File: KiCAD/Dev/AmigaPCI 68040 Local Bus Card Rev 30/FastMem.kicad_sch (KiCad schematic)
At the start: 29 parts, among them CN400 SPI, U400 ICE40HX1K-VQ100, U400F1 W25X20CLSN, U401 SDRAM(16Mx32), U402 SDRAM(16Mx32)

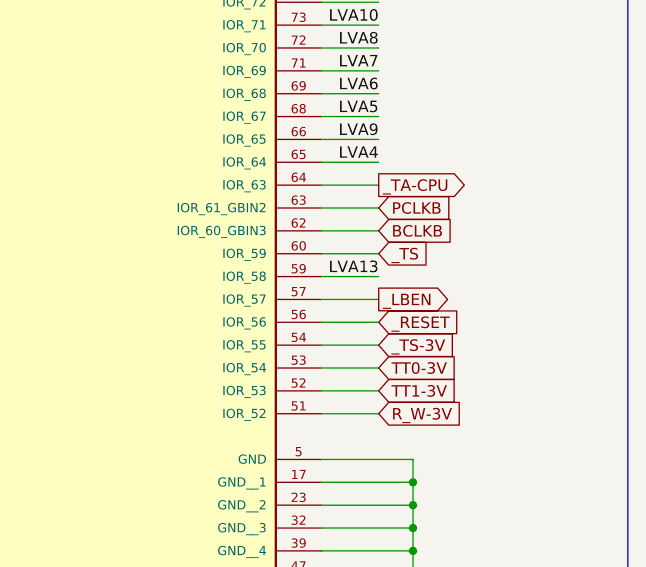
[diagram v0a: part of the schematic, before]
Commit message: CPU Local Bus Card Rev 3.0 Routing 18-JUL-2024
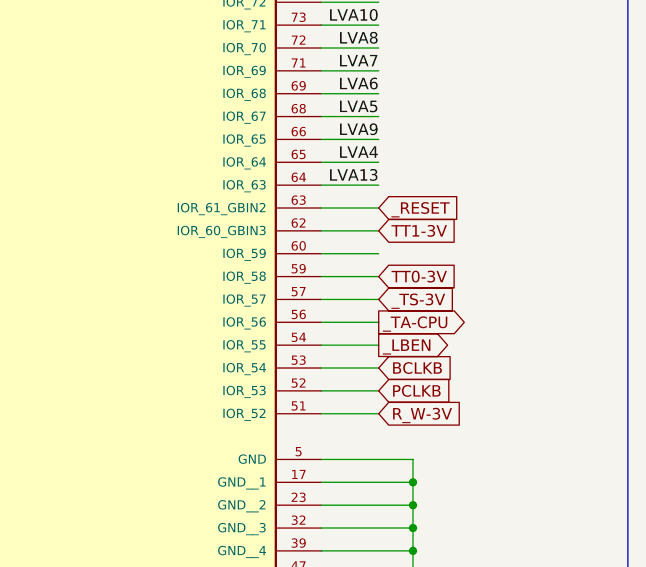
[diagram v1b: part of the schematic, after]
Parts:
- CN400: footprint Connector_PinHeader_2.54mm:PinHeader_2x03_P2.54mm_Vertical -> Connector_PinHeader_2.54mm:PinHeader_1x06_P2.54mm_Vertical
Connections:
- net BCLKB: now also U400.53 (IOR_54); no longer U400.62 (IOR_60_GBIN3)
- net LVA13: now also U400.64 (IOR_63); no longer U400.59 (IOR_58)
- net PCLKB: now also U400.52 (IOR_53); no longer U400.63 (IOR_61_GBIN2)
- net TT0-3V: now also U400.59 (IOR_58); no longer U400.53 (IOR_54)
- net TT1-3V: now also U400.62 (IOR_60_GBIN3); no longer U400.52 (IOR_53)
- net _LBEN: now also U400.54 (IOR_55); no longer U400.57 (IOR_57)
- net _RESET: now also U400.63 (IOR_61_GBIN2); no longer U400.56 (IOR_56)
- net _TA-CPU: now also U400.56 (IOR_56); no longer U400.64 (IOR_63)
- net _TS-3V: now also U400.57 (IOR_57); no longer U400.54 (IOR_55)
- net _TS: no longer names the net of U400.60 (IOR_59)
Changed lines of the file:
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@@
 	)
 	(label "LVA13"
-		(at 383.54 179.07 180)
+		(at 383.54 168.91 180)
 		(fields_autoplaced yes)
 		(effects
@@
 	(global_label "PCLKB"
 		(shape input)
-		(at 383.54 171.45 0)
+		(at 383.54 191.77 0)
 		(fields_autoplaced yes)
 		(effects
@@
 		)
 		(property "Intersheetrefs" "${INTERSHEET_REFS}"
-			(at 392.6333 171.45 0)
+			(at 392.6333 191.77 0)
 			(effects
 				(font
@@
 	(global_label "_TS-3V"
 		(shape input)
-		(at 383.54 186.69 0)
+		(at 383.54 181.61 0)
 		(fields_autoplaced yes)
 		(effects
@@
 		)
 		(property "Intersheetrefs" "${INTERSHEET_REFS}"
-			(at 393.5404 186.69 0)
+			(at 393.5404 181.61 0)
 			(effects
 				(font
@@
 	(global_label "TT1-3V"
 		(shape input)
-		(at 383.54 191.77 0)
+		(at 383.54 173.99 0)
 		(fields_autoplaced yes)
 		(effects
@@
 		)
 		(property "Intersheetrefs" "${INTERSHEET_REFS}"
-			(at 393.5404 191.77 0)
+			(at 393.5404 173.99 0)
 			(effects
 				(font
@@
 		)
 	)
-	(global_label "_TS"
-		(shape input)
-		(at 383.54 176.53 0)
+	(global_label "BANK1"
+		(shape input)
+		(at 158.75 118.11 180)
+		(fields_autoplaced yes)
+		(effects
+			(font
+				(size 1.27 1.27)
+			)
+			(justify right)
+		)
+		(property "Intersheetrefs" "${INTERSHEET_REFS}"
+			(at 149.5962 118.11 0)
+			(effects
+				(font
+					(size 1.27 1.27)
+				)
+				(justify right)
+			)
+		)
+	)
+	(global_label "TT0-3V"
+		(shape input)
+		(at 383.54 179.07 0)
 		(fields_autoplaced yes)
 		(effects
@@
 		)
 		(property "Intersheetrefs" "${INTERSHEET_REFS}"
-			(at 389.6699 176.53 0)
-			(effects
-				(font
-					(size 1.27 1.27)
-				)
-				(justify left)
-			)
-		)
-	)
-	(global_label "BANK1"
-		(shape input)
-		(at 158.75 118.11 180)
-		(fields_autoplaced yes)
-		(effects
-			(font
-				(size 1.27 1.27)
-			)
-			(justify right)
-		)
-		(property "Intersheetrefs" "${INTERSHEET_REFS}"
-			(at 149.5962 118.11 0)
-			(effects
-				(font
-					(size 1.27 1.27)
-				)
-				(justify right)
-			)
-		)
-	)
-	(global_label "TT0-3V"
-		(shape input)
-		(at 383.54 189.23 0)
-		(fields_autoplaced yes)
-		(effects
-			(font
-				(size 1.27 1.27)
-			)
-			(justify left)
-		)
-		(property "Intersheetrefs" "${INTERSHEET_REFS}"
-			(at 393.5404 189.23 0)
+			(at 393.5404 179.07 0)
 			(effects
 				(font
@@
 	(global_label "BCLKB"
 		(shape input)
-		(at 383.54 173.99 0)
+		(at 383.54 189.23 0)
 		(fields_autoplaced yes)
 		(effects
@@
 		)
 		(property "Intersheetrefs" "${INTERSHEET_REFS}"
-			(at 392.6333 173.99 0)
+			(at 392.6333 189.23 0)
 			(effects
 				(font
@@
 	(global_label "_TA-CPU"
 		(shape output)
-		(at 383.54 168.91 0)
+		(at 383.54 184.15 0)
 		(fields_autoplaced yes)
 		(effects
@@
 		)
 		(property "Intersheetrefs" "${INTERSHEET_REFS}"
-			(at 394.9919 168.91 0)
+			(at 394.9919 184.15 0)
 			(effects
 				(font
@@
 	(global_label "_RESET"
 		(shape input)
-		(at 383.54 184.15 0)
+		(at 383.54 171.45 0)
 		(fields_autoplaced yes)
 		(effects
@@
 		)
 		(property "Intersheetrefs" "${INTERSHEET_REFS}"
-			(at 393.2379 184.15 0)
+			(at 393.2379 171.45 0)
 			(effects
 				(font
@@
 	(global_label "_LBEN"
 		(shape output)
-		(at 383.54 181.61 0)
+		(at 383.54 186.69 0)
 		(fields_autoplaced yes)
 		(effects
@@
 		)
 		(property "Intersheetrefs" "${INTERSHEET_REFS}"
-			(at 392.2704 181.61 0)
+			(at 392.2704 186.69 0)
 			(effects
 				(font
@@
 			)
 		)
-		(property "Footprint" "Connector_PinHeader_2.54mm:PinHeader_2x03_P2.54mm_Vertical"
+		(property "Footprint" "Connector_PinHeader_2.54mm:PinHeader_1x06_P2.54mm_Vertical"
 			(at 262.89 74.93 0)
 			(effects
